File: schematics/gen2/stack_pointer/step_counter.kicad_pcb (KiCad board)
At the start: 2 copper layers, 87.5 x 104.1 mm, 16 parts, among them J1 Bus_PCI_Express_x16, U1 74LS00, U2 74LS193, U3 74LS193, U4 74LS193, U5 74LS193, U6 74LS245, U7 74LS245

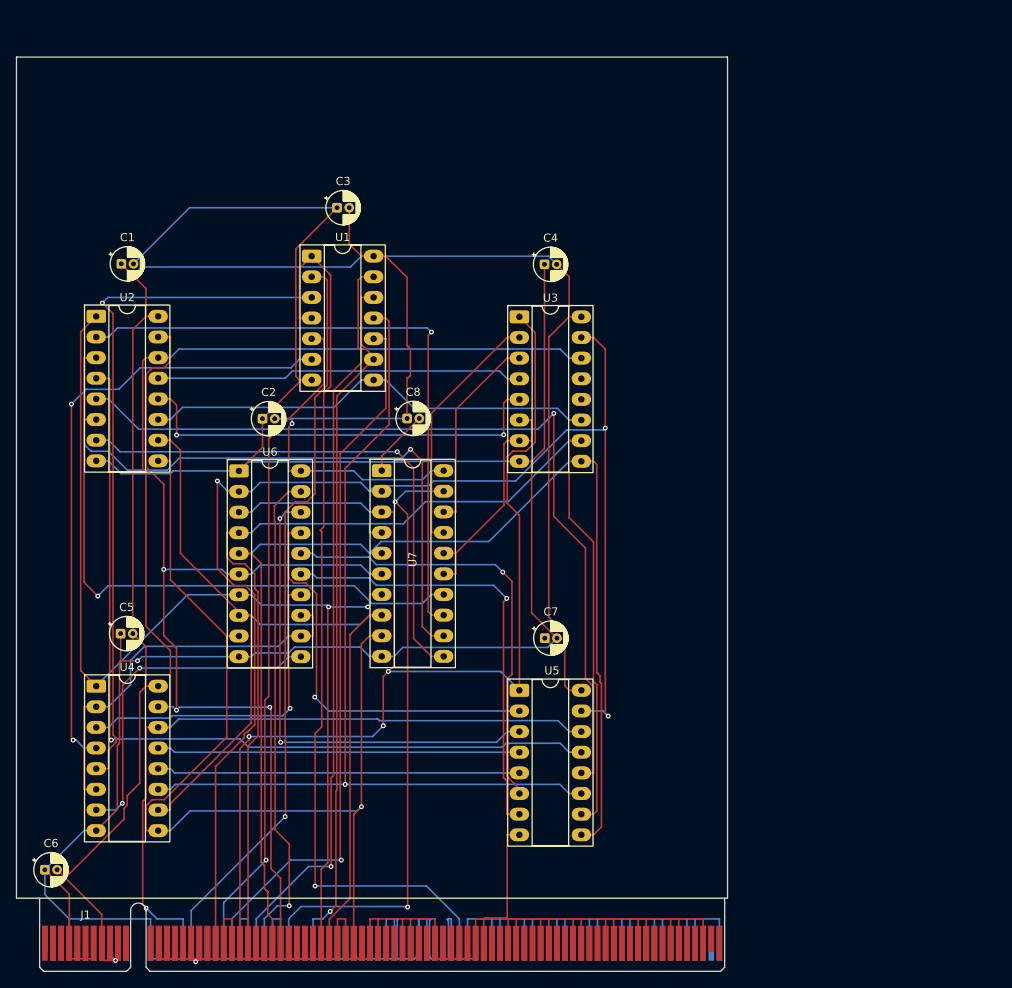
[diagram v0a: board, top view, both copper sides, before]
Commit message: (feat) step_counter update.
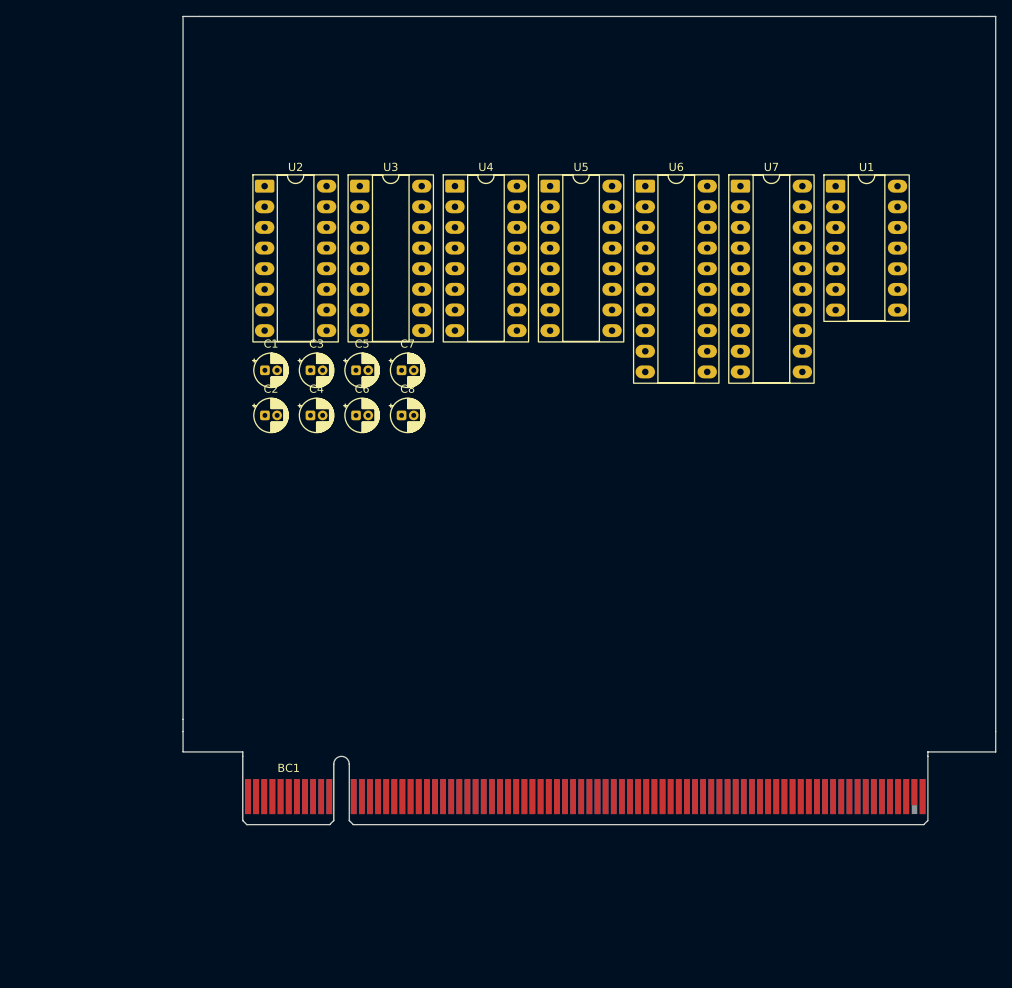
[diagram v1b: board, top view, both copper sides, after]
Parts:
- removed J1: Bus_PCI_Express_x16, Connector_PCBEdge:BUS_PCIexpress_x16
- added BC1: BusConnector, Connector_PCBEdge:BUS_PCIexpress_x16, F.Cu at (114.5, 130.0)
- moved U4 75.7 mm to (140.0, 54.9)
- moved C6 67.8 mm to (127.8, 83.1)
- moved U1 65.0 mm to (186.8, 54.9)
- moved U5 62.2 mm to (151.7, 54.9)
- moved U6 61.1 mm to (163.4, 54.9)
- moved U7 56.3 mm to (175.1, 54.9)
- moved C5 43.5 mm to (127.8, 77.5)
- moved C7 37.4 mm to (133.4, 77.5)
- moved C4 34.3 mm to (122.2, 83.1)
- moved U2 26.2 mm to (116.5, 54.9)
- moved U3 25.4 mm to (128.2, 54.9)
- moved C1 22.0 mm to (116.6, 77.5)
- moved C3 20.3 mm to (122.2, 77.5)
- moved C8 0.78 mm to (133.4, 83.1)
- moved C2 0.51 mm to (116.6, 83.1)
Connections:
- net /CPd_A renamed /CPd
- net /CPu_A renamed /CPu
- net /Ph_A renamed /Ph
- net /Pl_A renamed /Pl
- U1 pad 10: /PCHighIn -> /SPHighIn
- U1 pad 13: /PCLowIn -> /SPLowIn
- U1 pad 2: /PCInc -> /SPInc
- U1 pad 5: /PCDec -> /SPDec
- U3 pad 6: /DH3 -> /DH2
- U4 pad 2: /DL6 -> /DL5
- U6 pad 13: /DL6 -> /DL5
- U6 pad 19: /~{PCLowOut} -> /~{SPLowOut}
- U7 pad 16: /DH3 -> /DH2
- U7 pad 19: /~{PCHighOut} -> /~{SPHighOut}
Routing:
- net GND: track 668.0 -> 0.00 mm, vias 2 -> 0
- net VCC: track 298.2 -> 0.00 mm, vias 2 -> 0
- net /Reset: track 188.2 -> 0.00 mm, vias 1 -> 0
- net /BUS0: track 167.5 -> 0.00 mm, vias 3 -> 0
- net /BUS1: track 156.1 -> 0.00 mm, vias 3 -> 0
- net /BUS2: track 154.6 -> 0.00 mm
- net /BUS3: track 149.7 -> 0.00 mm
- net /BUS5: track 130.1 -> 0.00 mm, vias 2 -> 0
- net /BUS7: track 123.7 -> 0.00 mm, vias 1 -> 0
- net /BUS4: track 122.1 -> 0.00 mm, vias 3 -> 0
- net /BUS6: track 119.7 -> 0.00 mm
- net /Pl: track 114.1 -> 0.00 mm, vias 1 -> 0
- net /~{Clk}: track 111.2 -> 0.00 mm, vias 1 -> 0
- net Net-(U2-UP): track 106.4 -> 0.00 mm, vias 1 -> 0
- net Net-(U2-DOWN): track 105.1 -> 0.00 mm, vias 1 -> 0
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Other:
- board size 87.5 x 104.1 mm -> 100 x 91 mm

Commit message: pc and sp sch
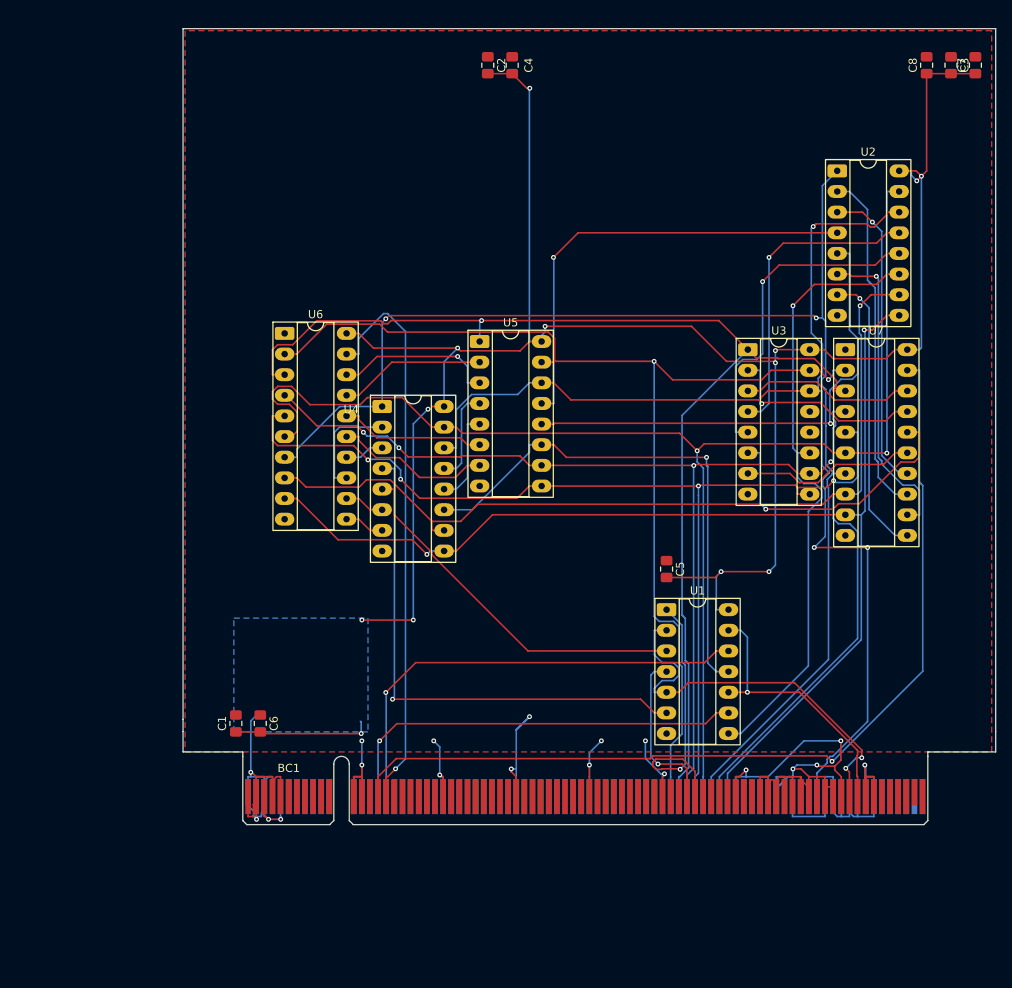
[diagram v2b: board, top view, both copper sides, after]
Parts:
- C1, C2, C3, C4, C5, C6, C7, C8: footprint Capacitor_THT:CP_Radial_D4.0mm_P1.50mm -> Capacitor_SMD:C_0805_2012Metric_Pad1.18x1.45mm_HandSolder
- moved C3 87.3 mm to (201.0, 40.0), turned to -90 degrees
- moved C7 80.0 mm to (204.0, 40.0), turned to 90 degrees
- moved C8 77.7 mm to (198.0, 40.0), turned to 90 degrees
- moved U2 70.5 mm to (187.0, 53.0)
- moved U1 56.1 mm to (166.0, 107.0)
- moved U3 51.8 mm to (176.0, 75.0)
- moved C2 51.1 mm to (144.0, 40.0), turned to -90 degrees
- moved C4 49.7 mm to (147.0, 40.0), turned to -90 degrees
- moved U6 47.9 mm to (119.0, 73.0)
- moved C5 45.4 mm to (166.0, 102.0), turned to -90 degrees
- moved C1 43.6 mm to (113.0, 121.0), turned to 90 degrees
- moved C6 39.7 mm to (116.0, 121.0), turned to -90 degrees
- moved U4 28.6 mm to (131.0, 82.0)
- moved U7 23.9 mm to (188.0, 75.0)
- moved U5 21.0 mm to (143.0, 74.0)
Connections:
- BC1 pad A15: unconnected-(BC1-LSPH-PadA15) -> /LSPH
- BC1 pad A16: unconnected-(BC1-LSPL-PadA16) -> /LSPL
- BC1 pad A21: /LAC -> unconnected-(BC1-~{LAC}-PadA21)
- BC1 pad A69: unconnected-(BC1-RESET-PadA69) -> /RESET
- BC1 pad B15: unconnected-(BC1-~{RSPH}-PadB15) -> /~{RSPH}
- BC1 pad B16: unconnected-(BC1-~{RSPL}-PadB16) -> /~{RSPL}
- BC1 pad B21: /~{RAC} -> unconnected-(BC1-~{RAC}-PadB21)
- BC1 pad B53: unconnected-(BC1-SPDEC-PadB53) -> /SPDEC
- BC1 pad B54: unconnected-(BC1-SPINC-PadB54) -> /SPINC
- BC1 pad B55: /ACSHLEFT -> unconnected-(BC1-ACSHLEFT-PadB55)
- BC1 pad B56: /ACSHRIGHT -> unconnected-(BC1-ACSHRIGHT-PadB56)
- BC1 pad B74: unconnected-(BC1-PULSE-PadB74) -> /PULSE
- U1 pad 1: /~{Clk} -> /SPINC
- U1 pad 10: /SPHighIn -> /PULSE
- U1 pad 12: /PULSE -> /LSPL
- U1 pad 13: /SPLowIn -> /PULSE
- U1 pad 2: /SPInc -> /~{CLK}
- U1 pad 4: /~{Clk} -> /SPDEC
- U1 pad 5: /SPDec -> /~{CLK}
- U1 pad 9: /PULSE -> /LSPH
- U2 pad 1: /BUS5 -> /DATA5
- U2 pad 10: /BUS6 -> /DATA6
- U2 pad 14: /Reset -> /RESET
- U2 pad 15: /BUS4 -> /DATA4
- U2 pad 9: /BUS7 -> /DATA7
- U3 pad 1: /BUS1 -> /DATA1
- U3 pad 10: /BUS2 -> /DATA2
- U3 pad 14: /Reset -> /RESET
- U3 pad 15: /BUS0 -> /DATA0
- U3 pad 9: /BUS3 -> /DATA3
- U4 pad 1: /BUS5 -> /DATA5
- U4 pad 10: /BUS6 -> /DATA6
- U4 pad 14: /Reset -> /RESET
- U4 pad 15: /BUS4 -> /DATA4
- U4 pad 9: /BUS7 -> /DATA7
- U5 pad 1: /BUS1 -> /DATA1
- U5 pad 10: /BUS2 -> /DATA2
- U5 pad 14: /Reset -> /RESET
- U5 pad 15: /BUS0 -> /DATA0
- U5 pad 9: /BUS3 -> /DATA3
- U6 pad 19: /~{SPLowOut} -> /~{RSPL}
- U6 pad 2: /BUS0 -> /DATA0
- U6 pad 3: /BUS1 -> /DATA1
- U6 pad 4: /BUS2 -> /DATA2
- U6 pad 5: /BUS3 -> /DATA3
- U6 pad 6: /BUS4 -> /DATA4
- U6 pad 7: /BUS5 -> /DATA5
- U6 pad 8: /BUS6 -> /DATA6
- U6 pad 9: /BUS7 -> /DATA7
- U7 pad 19: /~{SPHighOut} -> /~{RSPH}
- U7 pad 2: /BUS0 -> /DATA0
- U7 pad 3: /BUS1 -> /DATA1
- U7 pad 4: /BUS2 -> /DATA2
- U7 pad 5: /BUS3 -> /DATA3
- U7 pad 6: /BUS4 -> /DATA4
- U7 pad 7: /BUS5 -> /DATA5
- U7 pad 8: /BUS6 -> /DATA6
- U7 pad 9: /BUS7 -> /DATA7
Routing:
- net VCC: track 0.00 -> 325.6 mm, vias 0 -> 17
- net GND: track 0.00 -> 203.5 mm, vias 0 -> 15
- net /DATA5: track 0.00 -> 166.7 mm, vias 0 -> 2
- net /DATA4: track 0.00 -> 166.1 mm, vias 0 -> 2
- net /DATA6: track 0.00 -> 154.2 mm, vias 0 -> 1
- net /RESET: track 0.00 -> 147.4 mm, vias 0 -> 3
- net /DATA7: track 0.00 -> 145.3 mm, vias 0 -> 2
- net /DATA1: track 0.00 -> 144.2 mm, vias 0 -> 1
- net /DATA0: track 0.00 -> 135.0 mm, vias 0 -> 2
- net /DATA3: track 0.00 -> 129.4 mm, vias 0 -> 4
- net /DATA2: track 0.00 -> 121.3 mm, vias 0 -> 4
- net /~{RSPH}: track 0.00 -> 114.6 mm, vias 0 -> 1
- net /Ph: track 0.00 -> 76.8 mm, vias 0 -> 1
- net /~{RSPL}: track 0.00 -> 69.7 mm, vias 0 -> 1
- net /Pl: track 0.00 -> 65.4 mm, vias 0 -> 1
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- added copper zone on F.Cu, net GND
- added copper zone on B.Cu, net VCC
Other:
- board size 100 x 91 mm -> 100 x 89.5 mm
